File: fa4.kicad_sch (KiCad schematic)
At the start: 7 parts, among them U1 4081, U10 4071, U18 4069, U27 4069, U46 4071, U48 4081, U6 4081

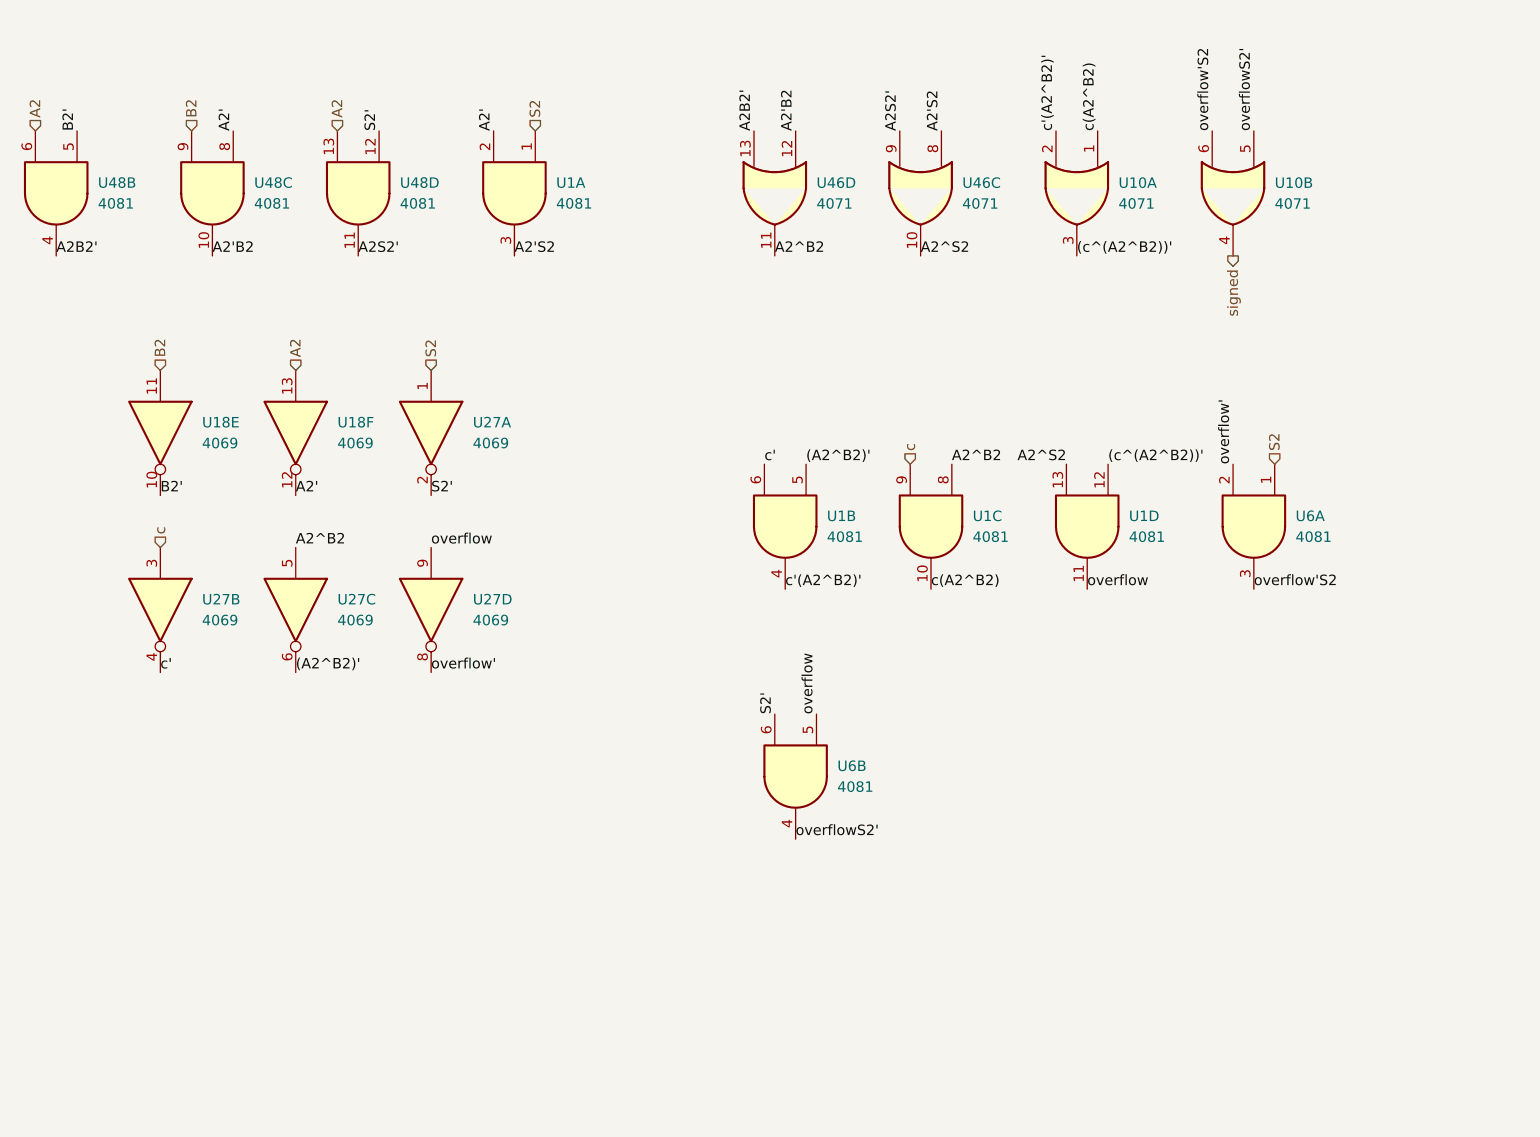
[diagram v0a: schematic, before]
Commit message: Add files via upload
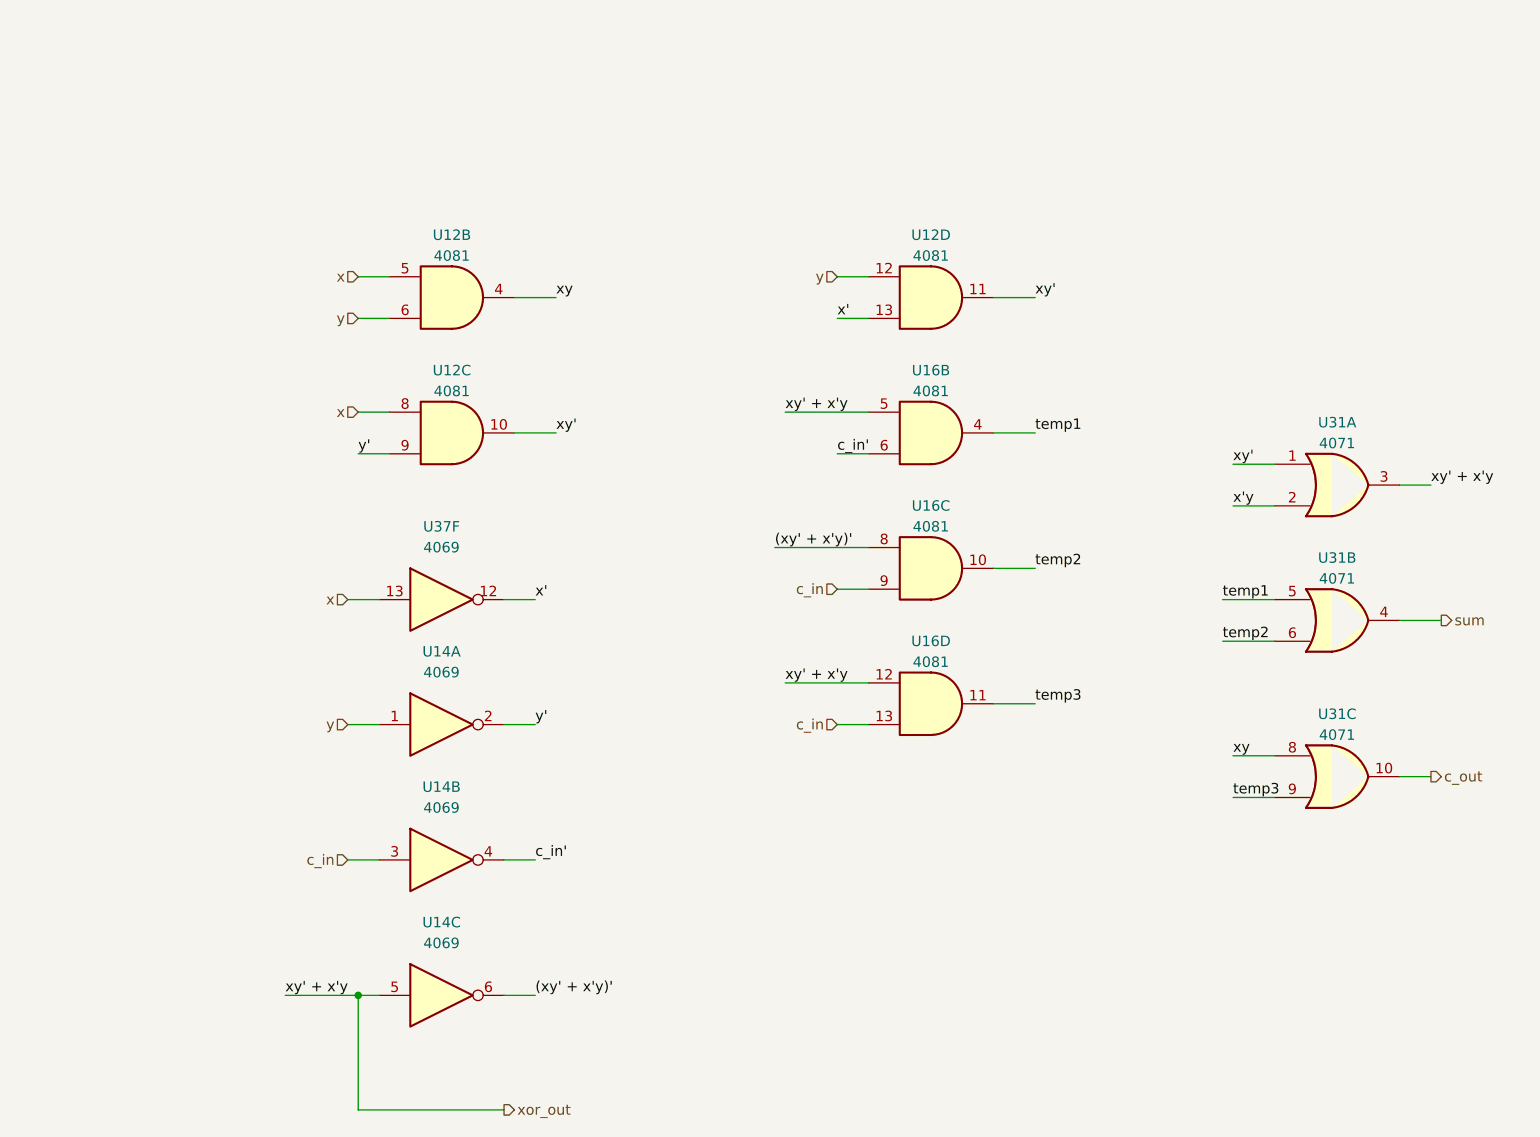
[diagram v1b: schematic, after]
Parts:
- removed U1, U48, U6: 4081, Package_DIP:CERDIP-14_W7.62mm_SideBrazed_LongPads_Socket, symbol 4xxx:4081
- removed U10, U46: 4071, Package_DIP:CERDIP-14_W7.62mm_SideBrazed_LongPads_Socket, symbol 4xxx:4071
- removed U18, U27: 4069, Package_DIP:CERDIP-14_W7.62mm_SideBrazed_LongPads_Socket, symbol 4xxx:4069
- added U12, U16: 4081, Package_DIP:CERDIP-14_W7.62mm_SideBrazed_LongPads_Socket, symbol 4xxx:4081
- added U14, U37: 4069, Package_DIP:CERDIP-14_W7.62mm_SideBrazed_LongPads_Socket, symbol 4xxx:4069
- added U31: 4071, Package_DIP:CERDIP-14_W7.62mm_SideBrazed_LongPads_Socket, symbol 4xxx:4071
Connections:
- new net (xy' + x'y)': U14.6, U16.8
- new net c_in: U14.3, U16.13, U16.9
- new net c_in': U14.4, U16.6
- new net c_out: U31.10
- new net sum: U31.4
- new net temp1: U16.4, U31.5
- new net temp2: U16.10, U31.6
- new net temp3: U16.11, U31.9
- new net x: U12.5, U12.8, U37.13
- new net x': U12.13, U37.12
- new net x'y: U31.2
- new net xor_out: U14.5, U16.12, U16.5, U31.3
- new net xy: U12.4, U31.8
- new net xy': U12.10, U12.11, U31.1
- new net y: U12.12, U12.6, U14.1
- new net y': U12.9, U14.2
